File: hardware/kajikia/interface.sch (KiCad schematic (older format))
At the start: 78 parts, among them J46 Conn_01x03, J47 Conn_01x03, J60 USB_C_Receptacle, J61 Micro_SD_Card_Det, J62 Conn_01x02, J63 Conn_01x02, J66 Conn_01x03, J67 Conn_01x03, J71 Conn_01x02, J72 Conn_01x02, J73 Conn_01x02, J74 Conn_01x02, Q2 AO3401, U5 MAX6675, U6 MAX6675

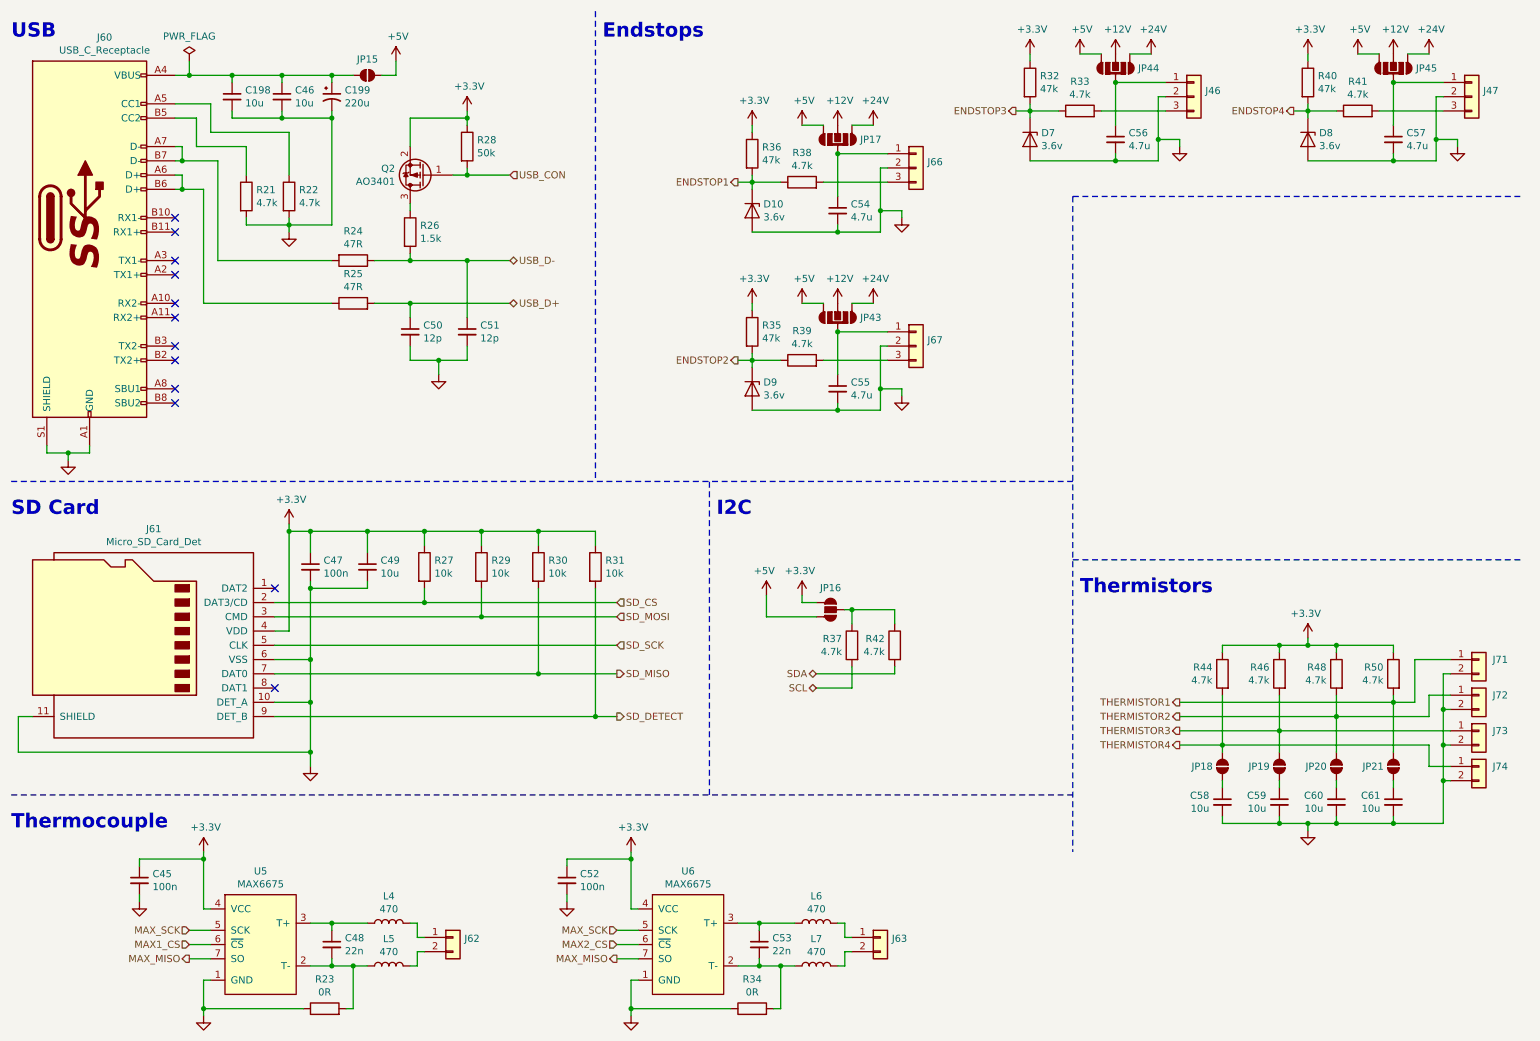
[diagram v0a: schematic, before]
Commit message: PCB V1
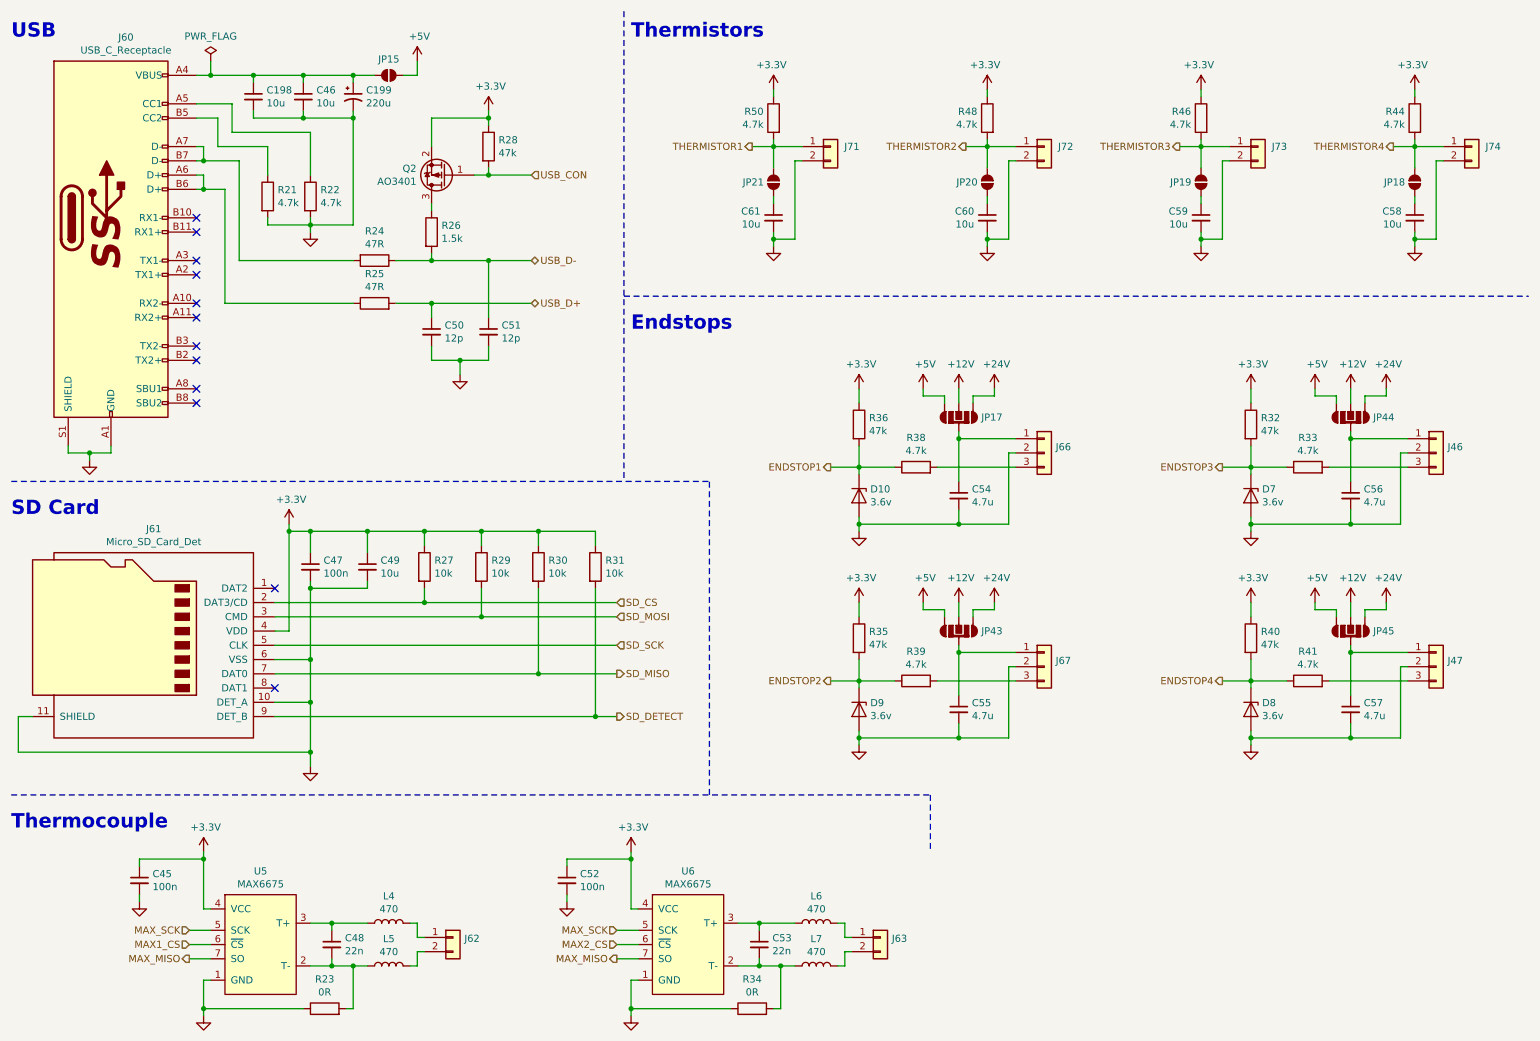
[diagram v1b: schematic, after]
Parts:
- removed JP16: SolderJumper_3_Open, _Generic:Solder Jumper 3P, symbol #PCB_Only:SolderJumper_3_Open
- removed R37, R42: 4.7k, _Generic:0603_RES, symbol Device:R
- R28: value 50k -> 47k
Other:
- note removed: "I2C"
- moved on the sheet: C198, C199, C46, C50, C51, C54, C55, C56, C57, C58, C59, C60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
